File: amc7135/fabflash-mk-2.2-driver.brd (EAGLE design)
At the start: 22 x 22 mm, 17 parts, among them Q1 MOSFET-PCHANNELIRLML2244, U1 LM2735YMF

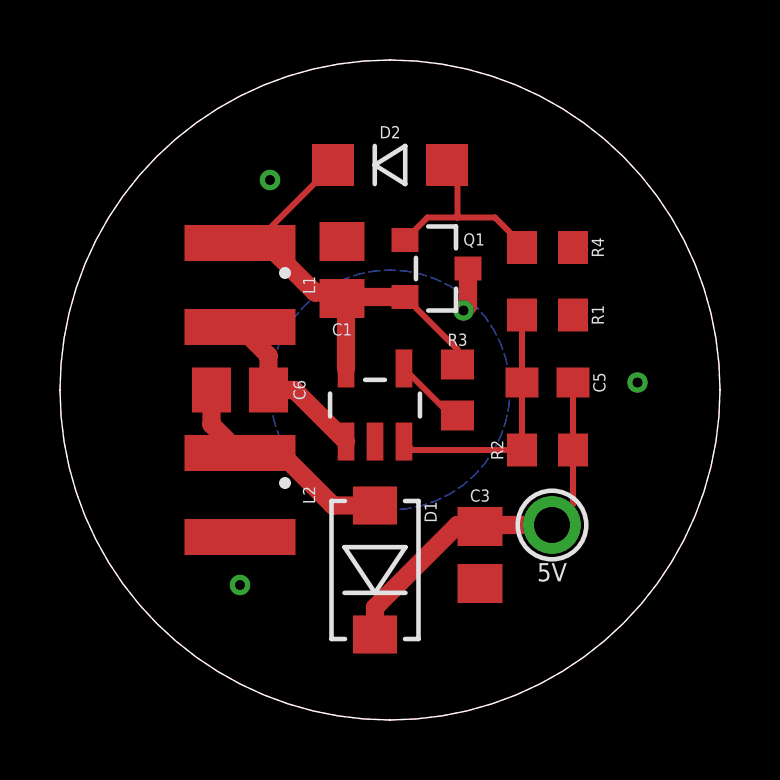
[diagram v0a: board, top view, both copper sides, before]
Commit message: two new tries at this, about to go for 3
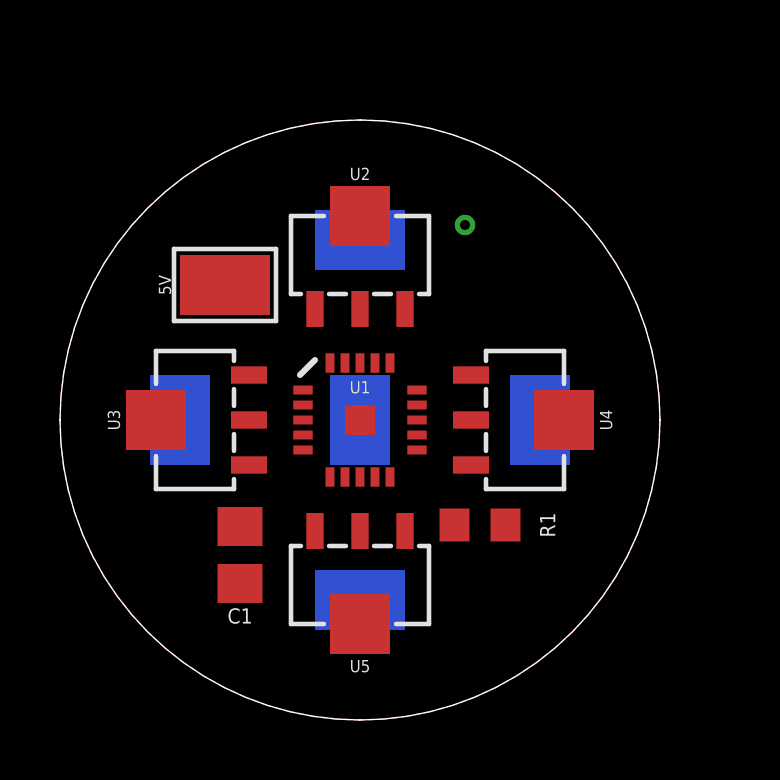
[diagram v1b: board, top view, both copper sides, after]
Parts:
- removed BATT+, BATT-: M01NOT-A-VIA-NOPE, A_butts:1X01_NOSILK_NOSTOP
- removed C3: 10uF, A_butts:C0805
- removed C5: 2.2nF, A_butts:C0603
- removed C6: 2.2uF, A_butts:C0805
- removed D1: B340A, A_butts:SMA-DIODE
- removed D2: 10V, A_butts:SOD123
- removed L1, L2: 6.8uH, A_butts:TAIYO-YUDEN-40XX
- removed Q1: MOSFET-PCHANNELIRLML2244, A_butts:SOT23-3
- removed R2: 30k, A_butts:R0603
- removed R3, R4: 100k, A_butts:R0603
- added +, B-, G-, R-, W-: M01SMD_2X3MM, A_butts:1X01_SMD_2X3MM
- added GND: M01NOT-A-VIA-NOPE, A_butts:1X01_NOSILK_NOSTOP
- added U2, U3, U4, U5: AMC7135SOT-89, A_butts:SOT89
- 5V: value M01PTH-1.2MM -> M01SMD_2X3MM; device A_butts:1X01-1.2MM -> A_butts:1X01_SMD_2X3MM
- C1: value 22uF -> 10uF
- R1: value 10k -> 100k
- U1: value LM2735YMF -> ATTINY84; device A_butts:SOT95P285X110-5N -> A_butts:QFN20
- moved 5V 13.5 mm to (5.50, 14.5), turned to 90 degrees
- moved C1 10.1 mm to (6.00, 5.50), turned to 270 degrees
- moved R1 7.35 mm to (14.0, 6.50), turned to 0 degrees
- moved U1 0.71 mm to (10.0, 10.0), turned to 0 degrees
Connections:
- removed net BATT+: BATT+.P$1, Q1.3
- removed net N$2: R3.2, U1.4
- removed net N$4: D2.A, Q1.1, R4.2
- removed net N$6: C6.2, D1.A, L2.1
- removed net N$8: C5.2, R1.2, R2.1, U1.3
- removed net VIN: C1.1, D2.C, L1.1, Q1.2, R3.1, U1.5
- removed net VOUT: 5V.P$1, C3.1, C5.1, D1.C, R2.2
- new net 5V: +.P$1, 5V.P$1, C1.1, R1.1, U1.9
- new net BLUE-: B-.P$1, U4.1
- new net BLUEPWM: U1.14, U4.3
- new net GREEN-: G-.P$1, U3.1
- new net GREENPWM: U1.16, U3.3
- new net RED-: R-.P$1, U2.1
- new net REDPWM: U1.15, U2.3
- new net WHITE-: U5.1, W-.P$1
- new net WHITEPWM: U1.20, U5.3
- net GND: now also GND.P$1, U1.8, U2.2, U2.4, U3.2, U3.4, U4.2, U4.4, U5.2, U5.4; no longer BATT-.P$1, C3.2, L2.2, R1.1, R4.1, U1.2
- net N$1: now also R1.2, U1.13; no longer C6.1, L1.2, U1.1
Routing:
- net VIN: track 15.3 -> 0.00 mm
- net VOUT: track 13.0 -> 0.00 mm
- net N$8: track 8.55 -> 0.00 mm
- net N$6: track 7.72 -> 0.00 mm
- net N$4: track 6.58 -> 0.00 mm
- net N$1: track 5.79 -> 0.00 mm
- net N$2: track 2.43 -> 0.00 mm
- net BATT+: track 1.46 -> 0.00 mm
- removed copper zone on layer 16, net BATT+
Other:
- board size 22 x 22 mm -> 20 x 20 mm
